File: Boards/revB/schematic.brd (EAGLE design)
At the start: 30 x 20 mm, 44 parts

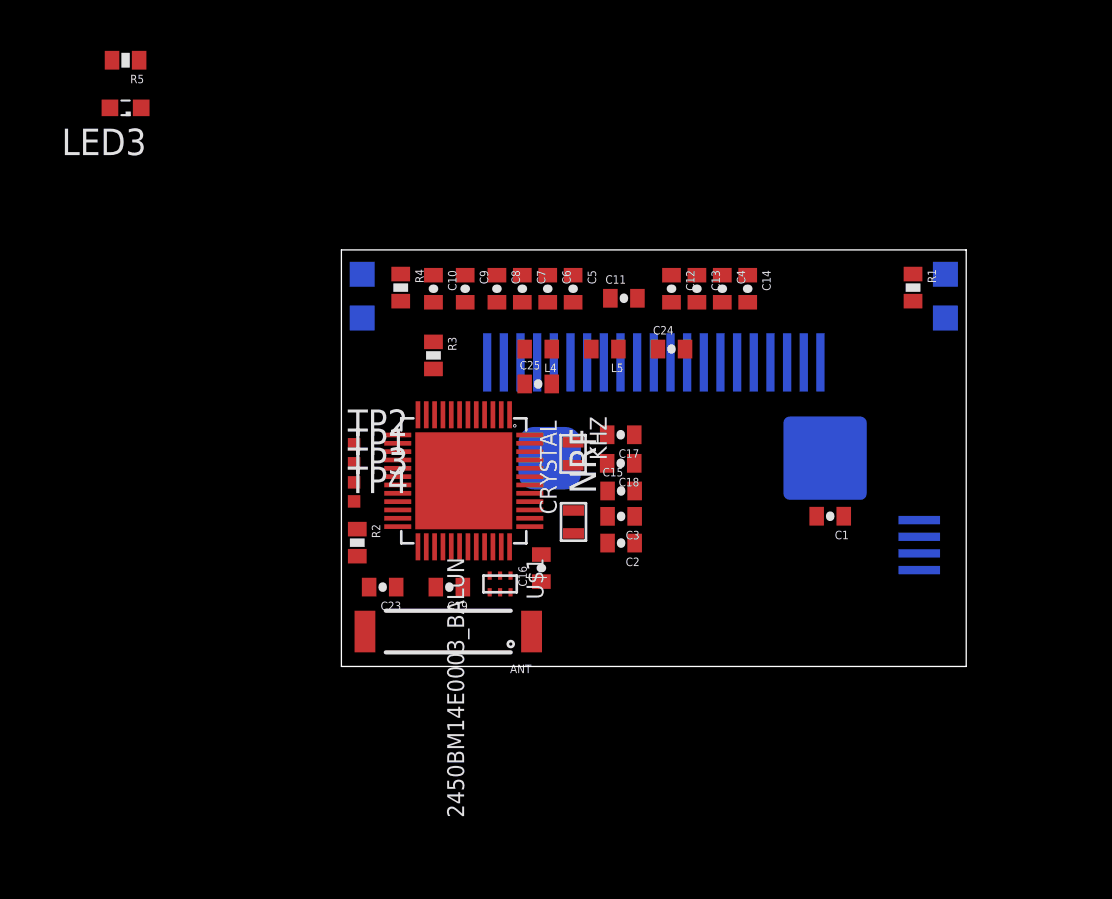
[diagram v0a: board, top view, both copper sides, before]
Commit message: LED ADDED and Component Placed.
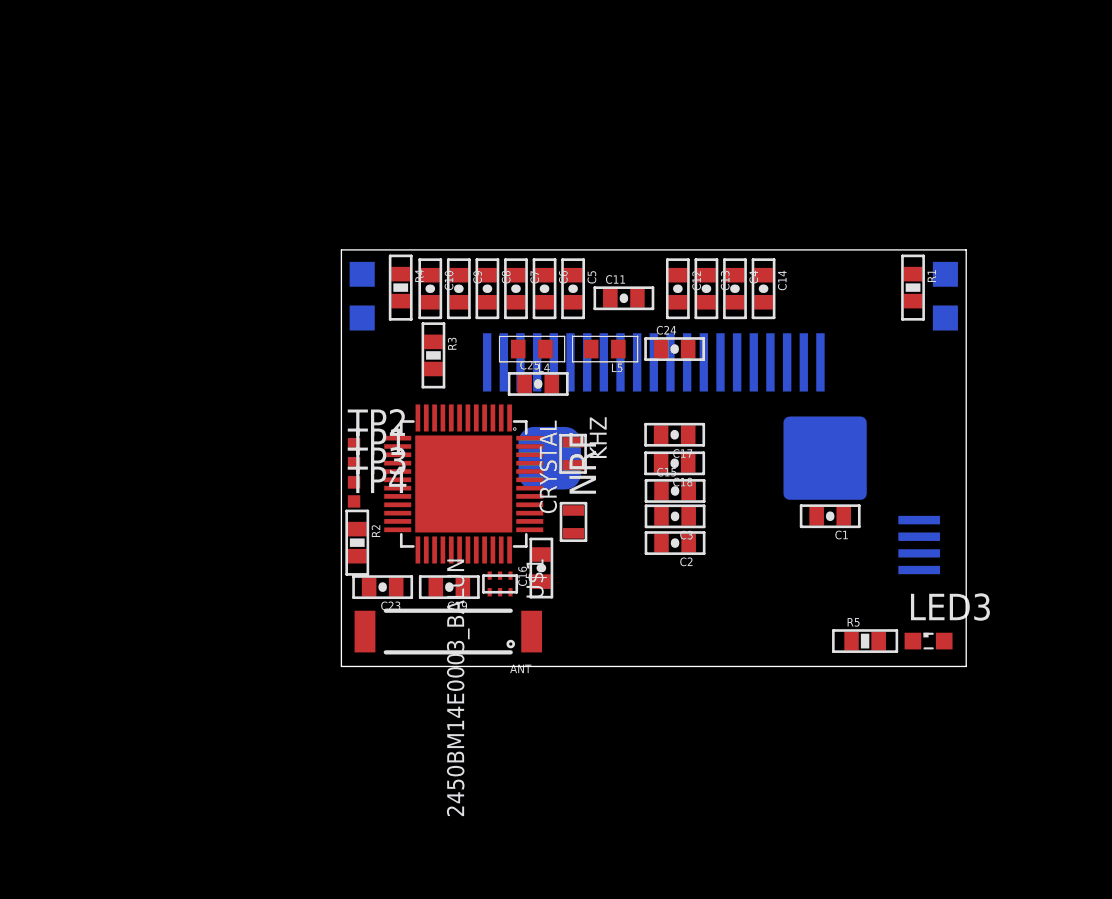
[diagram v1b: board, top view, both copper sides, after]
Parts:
- moved LED3 46.3 mm to (28.2, 1.22), turned to 0 degrees
- moved R5 45.2 mm to (25.1, 1.22), turned to 0 degrees
- moved C17 2.59 mm to (16.0, 11.1)
- moved C18 2.59 mm to (16.0, 9.75)
- moved C15 2.59 mm to (16.0, 8.43)
- moved C2 2.59 mm to (16.0, 5.93)
- moved C3 2.59 mm to (16.0, 7.21)
- moved C14 0.76 mm to (20.3, 18.1)
- moved C4 0.61 mm to (18.9, 18.1)
- moved C13 0.46 mm to (17.5, 18.1)
- moved C8 0.46 mm to (7.01, 18.1)
- moved C7 0.30 mm to (8.38, 18.1)
- moved C9 0.30 mm to (5.64, 18.1)
- moved L4 0.30 mm to (9.14, 15.2)
- moved C12 0.30 mm to (16.2, 18.1)
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
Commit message: Normal Push.
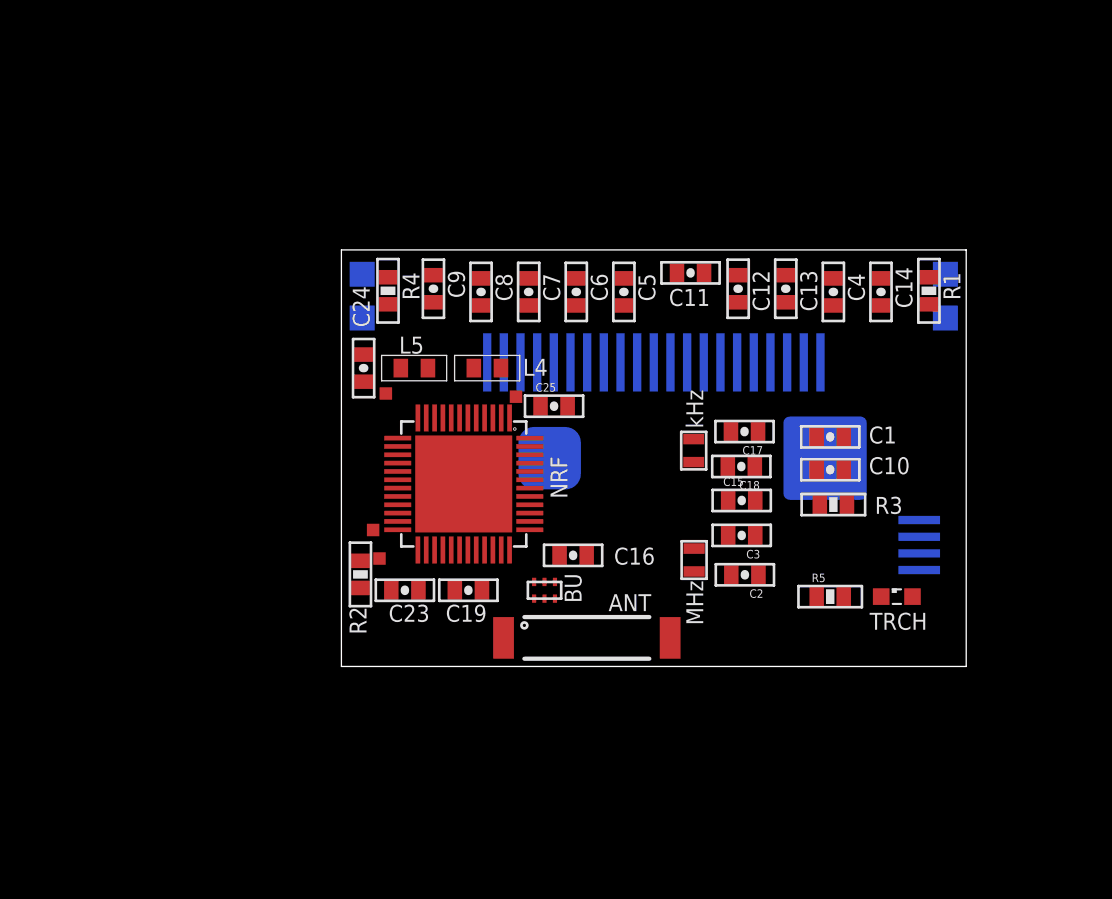
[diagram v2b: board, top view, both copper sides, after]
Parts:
- removed LED3: (no value), led:SML0603
- removed U$1: 2450BM14E0003_BALUN, baseOauth:6PCPADS
- added BU: 2450BM14E0003_BALUN, baseOauth:6PCPADS
- added TRCH: (no value), led:SML0603
- moved C10 21.1 mm to (23.5, 9.45), turned to 0 degrees
- moved R3 20.5 mm to (23.6, 7.77), turned to 180 degrees
- moved C24 15.0 mm to (1.07, 14.3), turned to 270 degrees
- moved L5 9.19 mm to (3.51, 14.3), turned to 0 degrees
- moved TP2 8.10 mm to (8.38, 13.0)
- moved ANT 6.66 mm to (11.8, 1.37), turned to 0 degrees
- moved 32MHZ 6.07 mm to (16.9, 5.11)
- moved KHZ 5.79 mm to (16.9, 10.4)
- moved C14 5.64 mm to (25.9, 18.0)
- moved C4 4.73 mm to (23.6, 18.0)
- moved C1 3.81 mm to (23.5, 11.0)
- moved C13 3.81 mm to (21.3, 18.1)
- moved C2 3.68 mm to (19.4, 4.40)
- moved TP1 3.68 mm to (2.13, 13.1)
- moved C11 3.42 mm to (16.8, 18.9)
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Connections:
- new net COG_IRS: LCD.P$1, NRF.25
- new net COG_RST: NRF.40, R3.2
- net ANT1: now also BU.P$3; no longer U$1.P$3
- net ANT2: now also BU.P$4; no longer U$1.P$4
- net FEED: now also BU.P$1; no longer U$1.P$1
- net GND: now also BU.P$2, BU.P$6, NRF.GND; no longer U$1.P$2, U$1.P$6
- net N$21: now also TRCH.C; no longer LED3.C
- net VDD: now also TRCH.A; no longer LED3.A
- net VDD_COG: no longer LCD.P$1, R3.2
- net VDD_PA: now also BU.P$5; no longer U$1.P$5
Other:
- board text added: "MHz"
- board text added: "kHz"

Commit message: Normal Push.
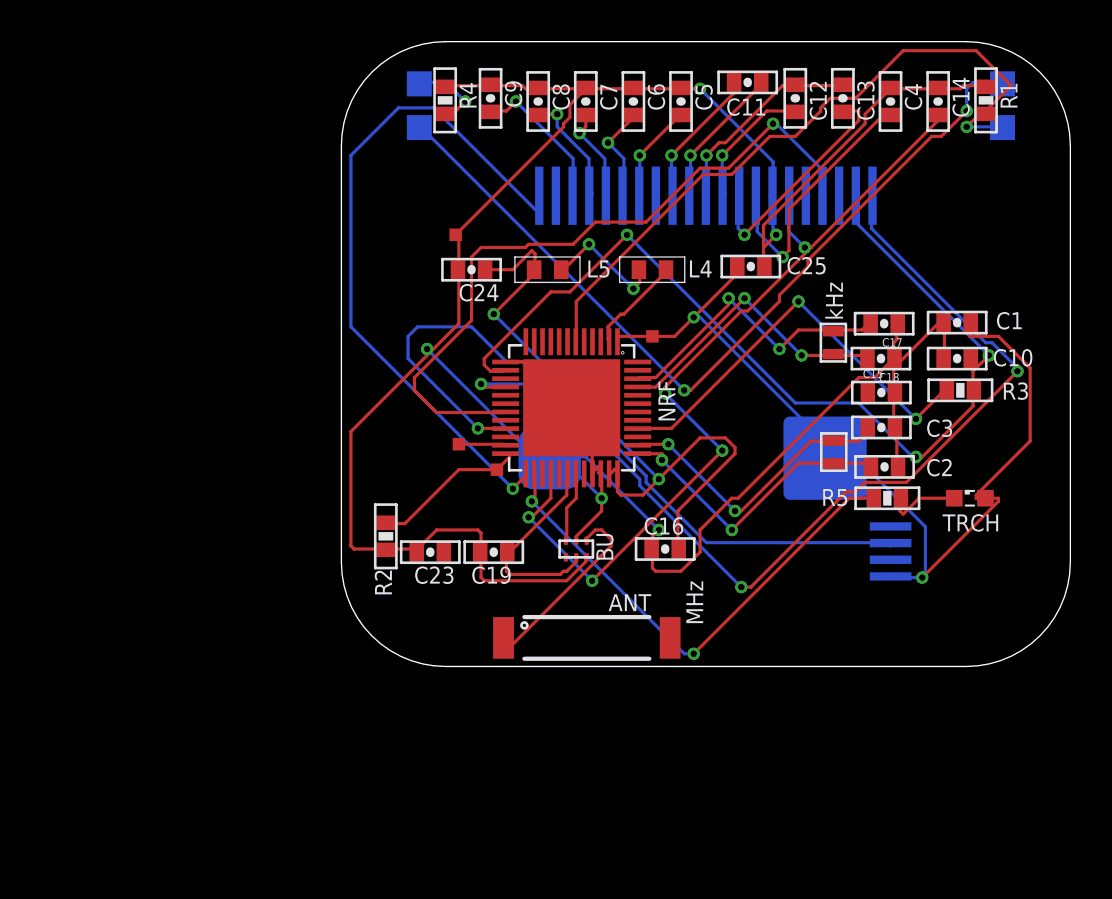
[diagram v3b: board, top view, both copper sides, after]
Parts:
- moved C25 11.6 mm to (19.7, 19.2)
- moved C11 9.55 mm to (19.5, 28.0)
- moved C13 9.55 mm to (24.1, 27.3)
- moved C4 9.55 mm to (26.4, 27.1)
- moved C5 9.55 mm to (16.3, 27.1)
- moved C6 9.55 mm to (14.0, 27.1)
- moved C7 9.55 mm to (11.7, 27.1)
- moved C8 9.55 mm to (9.45, 27.1)
- moved C9 9.55 mm to (7.16, 27.3)
- moved LED1 9.55 mm to (31.7, 26.9)
- moved LED2 9.55 mm to (3.74, 26.9)
- moved R1 9.55 mm to (31.0, 27.2)
- moved R4 9.55 mm to (4.98, 27.2)
- moved C12 9.55 mm to (21.8, 27.3)
- moved C14 9.55 mm to (28.7, 27.1)
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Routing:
- net GND: track 0.00 -> 145.7 mm, vias 0 -> 5
- net SS: track 0.00 -> 47.0 mm, vias 0 -> 3
- net RES: track 0.00 -> 47.0 mm, vias 0 -> 3
- net VDD: track 0.00 -> 46.6 mm, vias 0 -> 2
- net VDD_COG: track 0.00 -> 41.7 mm, vias 0 -> 5
- net VDD_PT: track 0.00 -> 40.5 mm, vias 0 -> 2
- net BTN2: track 0.00 -> 35.2 mm, vias 0 -> 1
- net SCK: track 0.00 -> 34.1 mm, vias 0 -> 1
- net DATA_L1: track 0.00 -> 33.5 mm, vias 0 -> 1
- net COG_IRS: track 0.00 -> 32.8 mm, vias 0 -> 1
- net AVDD: track 0.00 -> 32.6 mm, vias 0 -> 2
- net TORCHLED: track 0.00 -> 23.9 mm, vias 0 -> 2
- net COG_RST: track 0.00 -> 20.3 mm, vias 0 -> 2
- net N$17: track 0.00 -> 14.7 mm, vias 0 -> 2
- net N$14: track 0.00 -> 14.5 mm, vias 0 -> 2
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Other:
- board size 30 x 20 mm -> 35 x 30 mm
